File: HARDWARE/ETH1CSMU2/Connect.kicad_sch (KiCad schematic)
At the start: 8 parts, among them J301 C64AC, K301 HE3621A0510, K302 HE3621A0510, K303 HE3621A0510, K304 HE3621A0510, K305 HE3621A0510, U301 ULN2003A

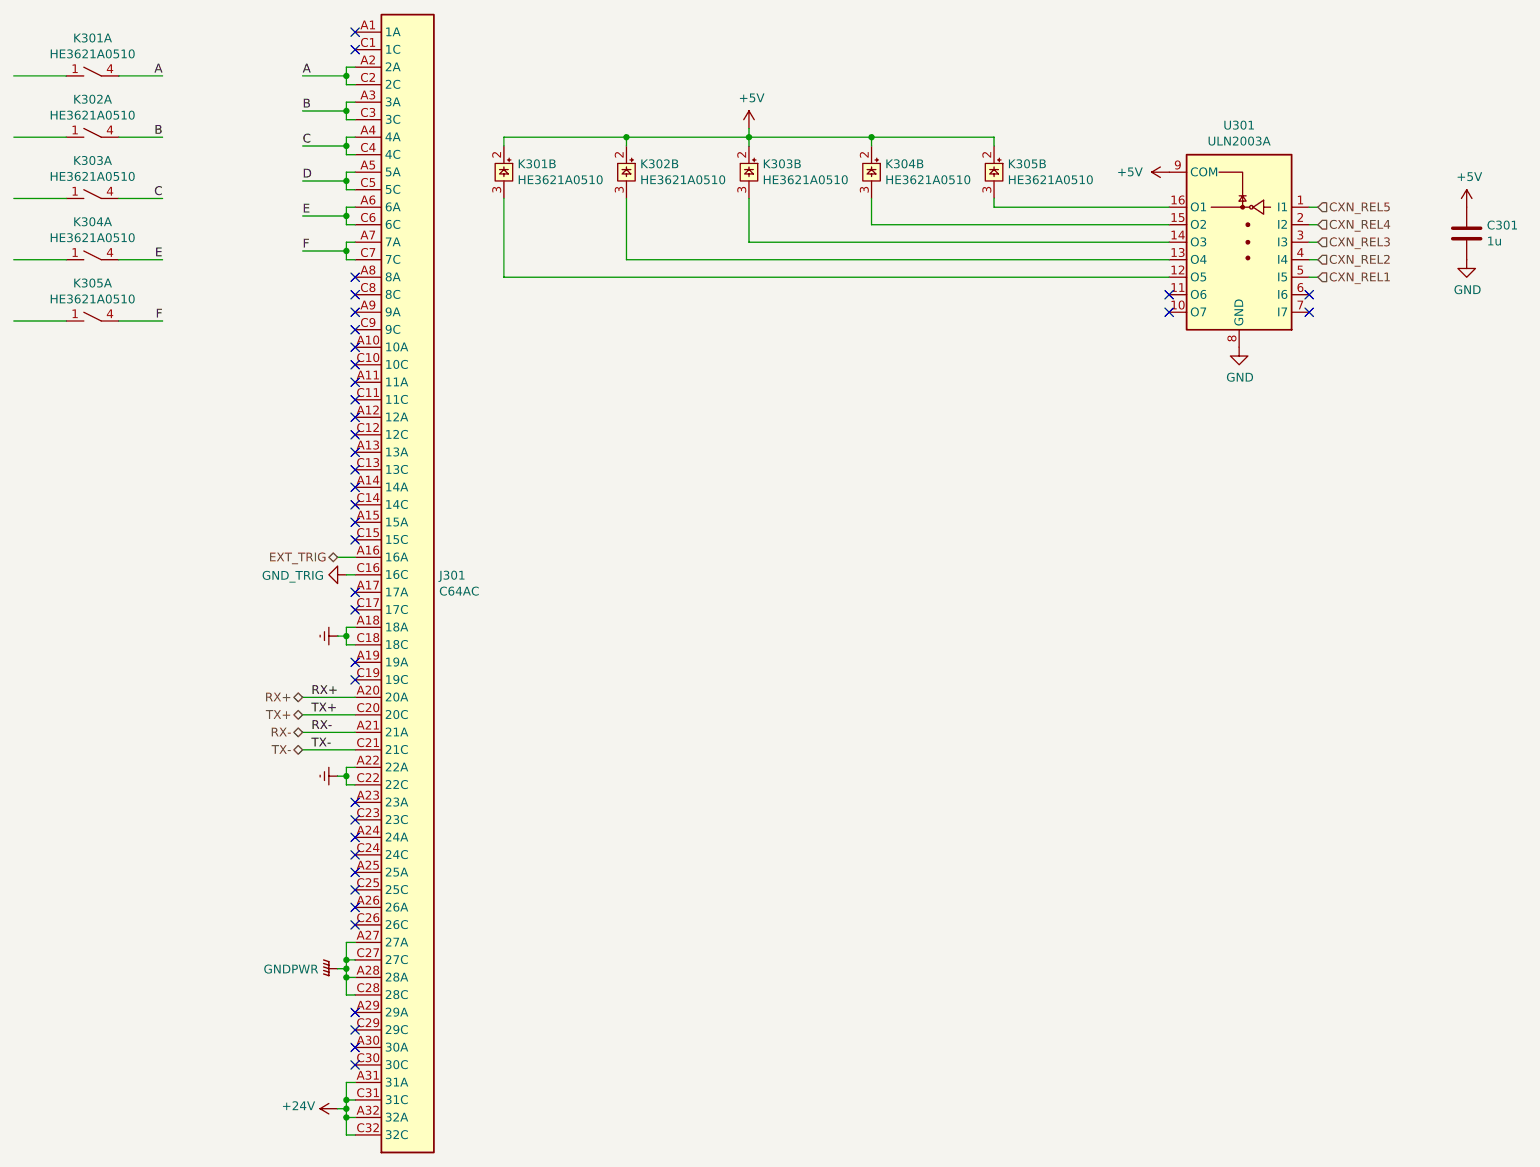
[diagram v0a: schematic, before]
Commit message: Hardware design
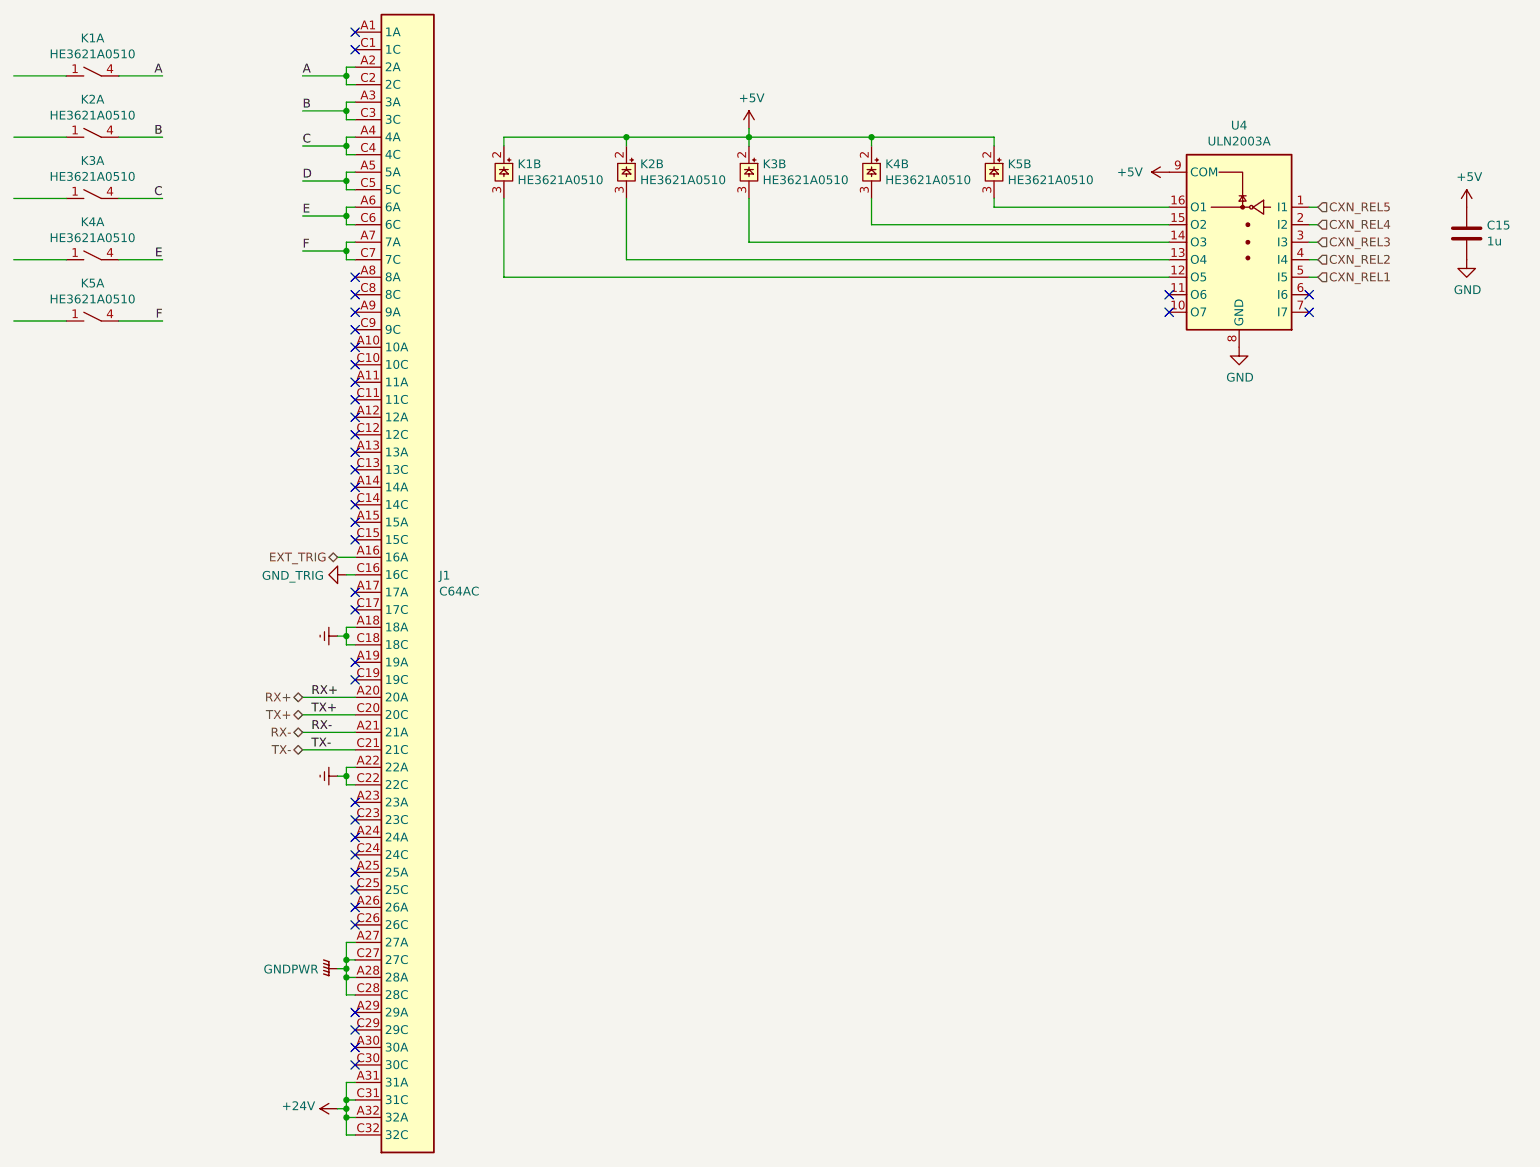
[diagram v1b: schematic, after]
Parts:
- renumbered C301 to C15, J301 to J1, K301 to K1, K302 to K2, K303 to K3, K304 to K4, K305 to K5, U301 to U4
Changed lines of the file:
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@@
   (symbol (lib_id "ETH1CSMU2:HE3621A0510") (at 77.47 58.42 90) (unit 1)
     (in_bom yes) (on_board yes)
-    (property "Reference" "K304" (id 0) (at 77.47 52.959 90))
+    (property "Reference" "K4" (id 0) (at 77.47 52.959 90))
     (property "Value" "HE3621A0510" (id 1) (at 77.47 55.2704 90))
     (property "Footprint" "ETH1CSMU1:HE360_x-5050462-8" (id 2) (at 78.74 52.07 0)
@@
   (symbol (lib_id "power:+24V") (at 113.03 181.61 90) (unit 1)
     (in_bom yes) (on_board yes)
-    (property "Reference" "#PWR0304" (id 0) (at 116.84 181.61 0)
+    (property "Reference" "#PWR027" (id 0) (at 116.84 181.61 0)
       (effects (font (size 1.27 1.27)) hide)
     )
@@
   (symbol (lib_id "Transistor_Array:ULN2003A") (at 243.84 55.88 0) (mirror y) (unit 1)
     (in_bom yes) (on_board yes)
-    (property "Reference" "U301" (id 0) (at 243.84 38.9382 0))
+    (property "Reference" "U4" (id 0) (at 243.84 38.9382 0))
     (property "Value" "ULN2003A" (id 1) (at 243.84 41.2496 0))
     (property "Footprint" "Package_SO:TSSOP-16_4.4x5mm_P0.65mm" (id 2) (at 242.57 69.85 0)
@@
   (symbol (lib_id "ETH1CSMU2:HE3621A0510") (at 77.47 67.31 90) (unit 1)
     (in_bom yes) (on_board yes)
-    (property "Reference" "K305" (id 0) (at 77.47 61.849 90))
+    (property "Reference" "K5" (id 0) (at 77.47 61.849 90))
     (property "Value" "HE3621A0510" (id 1) (at 77.47 64.1604 90))
     (property "Footprint" "ETH1CSMU1:HE360_x-5050462-8" (id 2) (at 78.74 60.96 0)
@@
   (symbol (lib_id "ETH1CSMU2:HE3621A0510") (at 208.28 45.72 0) (unit 2)
     (in_bom yes) (on_board yes)
-    (property "Reference" "K305" (id 0) (at 210.2612 44.5516 0)
+    (property "Reference" "K5" (id 0) (at 210.2612 44.5516 0)
       (effects (font (size 1.27 1.27)) (justify left))
     )
@@
   (symbol (lib_id "ETH1CSMU2:HE3621A0510") (at 77.47 40.64 90) (unit 1)
     (in_bom yes) (on_board yes)
-    (property "Reference" "K302" (id 0) (at 77.47 35.179 90))
+    (property "Reference" "K2" (id 0) (at 77.47 35.179 90))
     (property "Value" "HE3621A0510" (id 1) (at 77.47 37.4904 90))
     (property "Footprint" "ETH1CSMU1:HE360_x-5050462-8" (id 2) (at 78.74 34.29 0)
@@
   (symbol (lib_id "ETH1CSMU2:HE3621A0510") (at 77.47 49.53 90) (unit 1)
     (in_bom yes) (on_board yes)
-    (property "Reference" "K303" (id 0) (at 77.47 44.069 90))
+    (property "Reference" "K3" (id 0) (at 77.47 44.069 90))
     (property "Value" "HE3621A0510" (id 1) (at 77.47 46.3804 90))
     (property "Footprint" "ETH1CSMU1:HE360_x-5050462-8" (id 2) (at 78.74 43.18 0)
@@
   (symbol (lib_id "ETH1CSMU2:HE3621A0510") (at 172.72 45.72 0) (unit 2)
     (in_bom yes) (on_board yes)
-    (property "Reference" "K303" (id 0) (at 174.7012 44.5516 0)
+    (property "Reference" "K3" (id 0) (at 174.7012 44.5516 0)
       (effects (font (size 1.27 1.27)) (justify left))
     )
@@
   (symbol (lib_id "power:+5V") (at 172.72 39.37 0) (unit 1)
     (in_bom yes) (on_board yes)
-    (property "Reference" "#PWR0306" (id 0) (at 172.72 43.18 0)
+    (property "Reference" "#PWR029" (id 0) (at 172.72 43.18 0)
       (effects (font (size 1.27 1.27)) hide)
     )
@@
   (symbol (lib_id "ETH1CSMU2:HE3621A0510") (at 137.16 45.72 0) (unit 2)
     (in_bom yes) (on_board yes)
-    (property "Reference" "K301" (id 0) (at 139.1412 44.5516 0)
+    (property "Reference" "K1" (id 0) (at 139.1412 44.5516 0)
       (effects (font (size 1.27 1.27)) (justify left))
     )
@@
   (symbol (lib_id "power:GND") (at 243.84 71.12 0) (unit 1)
     (in_bom yes) (on_board yes)
-    (property "Reference" "#PWR0308" (id 0) (at 243.84 77.47 0)
+    (property "Reference" "#PWR031" (id 0) (at 243.84 77.47 0)
       (effects (font (size 1.27 1.27)) hide)
     )
@@
   (symbol (lib_id "power:GNDPWR") (at 113.03 161.29 270) (unit 1)
     (in_bom yes) (on_board yes)
-    (property "Reference" "#PWR0303" (id 0) (at 107.95 161.29 0)
+    (property "Reference" "#PWR026" (id 0) (at 107.95 161.29 0)
       (effects (font (size 1.27 1.27)) hide)
     )
@@
   (symbol (lib_id "power:Earth") (at 113.03 133.35 270) (unit 1)
     (in_bom yes) (on_board yes)
-    (property "Reference" "#PWR0302" (id 0) (at 106.68 133.35 0)
+    (property "Reference" "#PWR025" (id 0) (at 106.68 133.35 0)
       (effects (font (size 1.27 1.27)) hide)
     )
@@
   (symbol (lib_id "ETH1CSMU2:HE3621A0510") (at 190.5 45.72 0) (unit 2)
     (in_bom yes) (on_board yes)
-    (property "Reference" "K304" (id 0) (at 192.4812 44.5516 0)
+    (property "Reference" "K4" (id 0) (at 192.4812 44.5516 0)
       (effects (font (size 1.27 1.27)) (justify left))
     )
@@
   (symbol (lib_id "power:Earth") (at 113.03 113.03 270) (unit 1)
     (in_bom yes) (on_board yes)
-    (property "Reference" "#PWR0301" (id 0) (at 106.68 113.03 0)
+    (property "Reference" "#PWR024" (id 0) (at 106.68 113.03 0)
       (effects (font (size 1.27 1.27)) hide)
     )
@@
   (symbol (lib_id "Device:C") (at 276.86 54.61 0) (unit 1)
     (in_bom yes) (on_board yes)
-    (property "Reference" "C301" (id 0) (at 279.781 53.4416 0)
+    (property "Reference" "C15" (id 0) (at 279.781 53.4416 0)
       (effects (font (size 1.27 1.27)) (justify left))
     )
@@
   (symbol (lib_id "power:GND") (at 276.86 58.42 0) (unit 1)
     (in_bom yes) (on_board yes)
-    (property "Reference" "#PWR0310" (id 0) (at 276.86 64.77 0)
+    (property "Reference" "#PWR033" (id 0) (at 276.86 64.77 0)
       (effects (font (size 1.27 1.27)) hide)
     )
@@
   (symbol (lib_id "ETH1CSMU2:GND_TRIG") (at 114.3 104.14 270) (unit 1)
     (in_bom yes) (on_board yes)
-    (property "Reference" "#PWR0305" (id 0) (at 107.95 104.14 0)
+    (property "Reference" "#PWR028" (id 0) (at 107.95 104.14 0)
       (effects (font (size 1.27 1.27)) hide)
     )
@@
   (symbol (lib_id "power:+5V") (at 233.68 45.72 90) (unit 1)
     (in_bom yes) (on_board yes)
-    (property "Reference" "#PWR0307" (id 0) (at 237.49 45.72 0)
+    (property "Reference" "#PWR030" (id 0) (at 237.49 45.72 0)
       (effects (font (size 1.27 1.27)) hide)
     )
@@
   (symbol (lib_id "Connector:C64AC") (at 123.19 106.68 0) (unit 1)
     (in_bom yes) (on_board yes)
-    (property "Reference" "J301" (id 0) (at 127.762 104.2416 0)
+    (property "Reference" "J1" (id 0) (at 127.762 104.2416 0)
       (effects (font (size 1.27 1.27)) (justify left))
     )
@@
   (symbol (lib_id "power:+5V") (at 276.86 50.8 0) (unit 1)
     (in_bom yes) (on_board yes)
-    (property "Reference" "#PWR0309" (id 0) (at 276.86 54.61 0)
+    (property "Reference" "#PWR032" (id 0) (at 276.86 54.61 0)
       (effects (font (size 1.27 1.27)) hide)
     )
@@
   (symbol (lib_id "ETH1CSMU2:HE3621A0510") (at 154.94 45.72 0) (unit 2)
     (in_bom yes) (on_board yes)
-    (property "Reference" "K302" (id 0) (at 156.9212 44.5516 0)
+    (property "Reference" "K2" (id 0) (at 156.9212 44.5516 0)
       (effects (font (size 1.27 1.27)) (justify left))
     )
@@
   (symbol (lib_id "ETH1CSMU2:HE3621A0510") (at 77.47 31.75 90) (unit 1)
     (in_bom yes) (on_board yes)
-    (property "Reference" "K301" (id 0) (at 77.47 26.289 90))
+    (property "Reference" "K1" (id 0) (at 77.47 26.289 90))
     (property "Value" "HE3621A0510" (id 1) (at 77.47 28.6004 90))
     (property "Footprint" "ETH1CSMU1:HE360_x-5050462-8" (id 2) (at 78.74 25.4 0)
